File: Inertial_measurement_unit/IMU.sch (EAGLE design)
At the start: 16 parts, among them IC1 BNO055, Y1 ECS-.327-12.5-39-TR

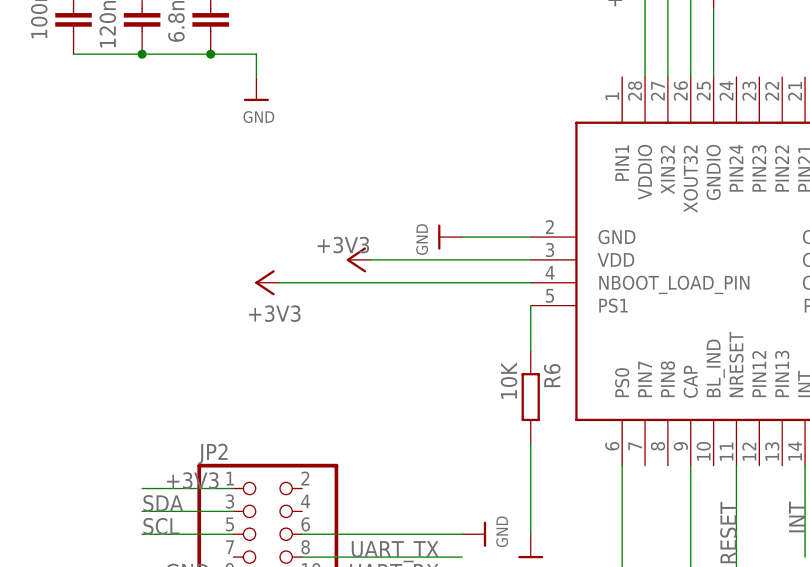
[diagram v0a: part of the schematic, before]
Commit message: Fixed traces, added BOM
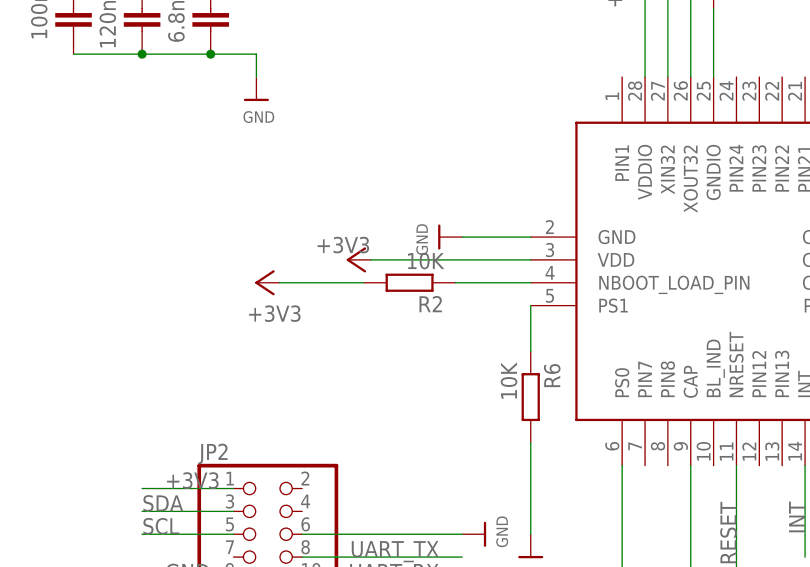
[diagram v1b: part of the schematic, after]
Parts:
- added R2: 10K, resistor:R-EU_R0805
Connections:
- new net NBOOT: IC1.NBOOT_LOAD_PIN, R2.1
- net +3V3: now also R2.2; no longer IC1.NBOOT_LOAD_PIN
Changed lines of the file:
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@@
 <part name="U$13" library="Airquality_Sensor" library_urn="urn:adsk.eagle:library:16015176" deviceset="GND" device=""/>
 <part name="JP1" library="pinhead" library_urn="urn:adsk.eagle:library:325" deviceset="PINHD-1X4" device="" package3d_urn="urn:adsk.eagle:package:22407/2"/>
+<part name="R2" library="resistor" library_urn="urn:adsk.eagle:library:348" deviceset="R-EU_" device="R0805" package3d_urn="urn:adsk.eagle:package:23553/2" value="10K"/>
 </parts>
 <sheets>
@@
 <attribute name="VALUE" x="16.51" y="38.1" size="1.778" layer="96"/>
 </instance>
+<instance part="R2" gate="G$1" x="-18.542" y="121.92" smashed="yes" rot="R180">
+<attribute name="NAME" x="-14.732" y="120.4214" size="1.778" layer="95" rot="R180"/>
+<attribute name="VALUE" x="-14.732" y="125.222" size="1.778" layer="96" rot="R180"/>
+</instance>
 </instances>
 <busses>
@@
 </segment>
 <segment>
-<pinref part="+3V4" gate="G$1" pin="+3V3"/>
-<pinref part="IC1" gate="G$1" pin="NBOOT_LOAD_PIN"/>
-<wire x1="-33.02" y1="121.92" x2="-5.08" y2="121.92" width="0.1524" layer="91"/>
-</segment>
-<segment>
 <pinref part="R1" gate="G$1" pin="2"/>
 <wire x1="76.2" y1="162.56" x2="76.2" y2="167.64" width="0.1524" layer="91"/>
@@
 <wire x1="86.36" y1="162.56" x2="86.36" y2="167.64" width="0.1524" layer="91"/>
 </segment>
+<segment>
+<pinref part="R2" gate="G$1" pin="2"/>
+<pinref part="+3V4" gate="G$1" pin="+3V3"/>
+<wire x1="-23.622" y1="121.92" x2="-33.02" y2="121.92" width="0.1524" layer="91"/>
+</segment>
 </net>
 <net name="CAP" class="0">
@@
 </segment>
 </net>
+<net name="NBOOT" class="0">
+<segment>
+<pinref part="IC1" gate="G$1" pin="NBOOT_LOAD_PIN"/>
+<pinref part="R2" gate="G$1" pin="1"/>
+<wire x1="-5.08" y1="121.92" x2="-13.462" y2="121.92" width="0.1524" layer="91"/>
+</segment>
+</net>
